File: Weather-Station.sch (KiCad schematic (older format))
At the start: 61 parts

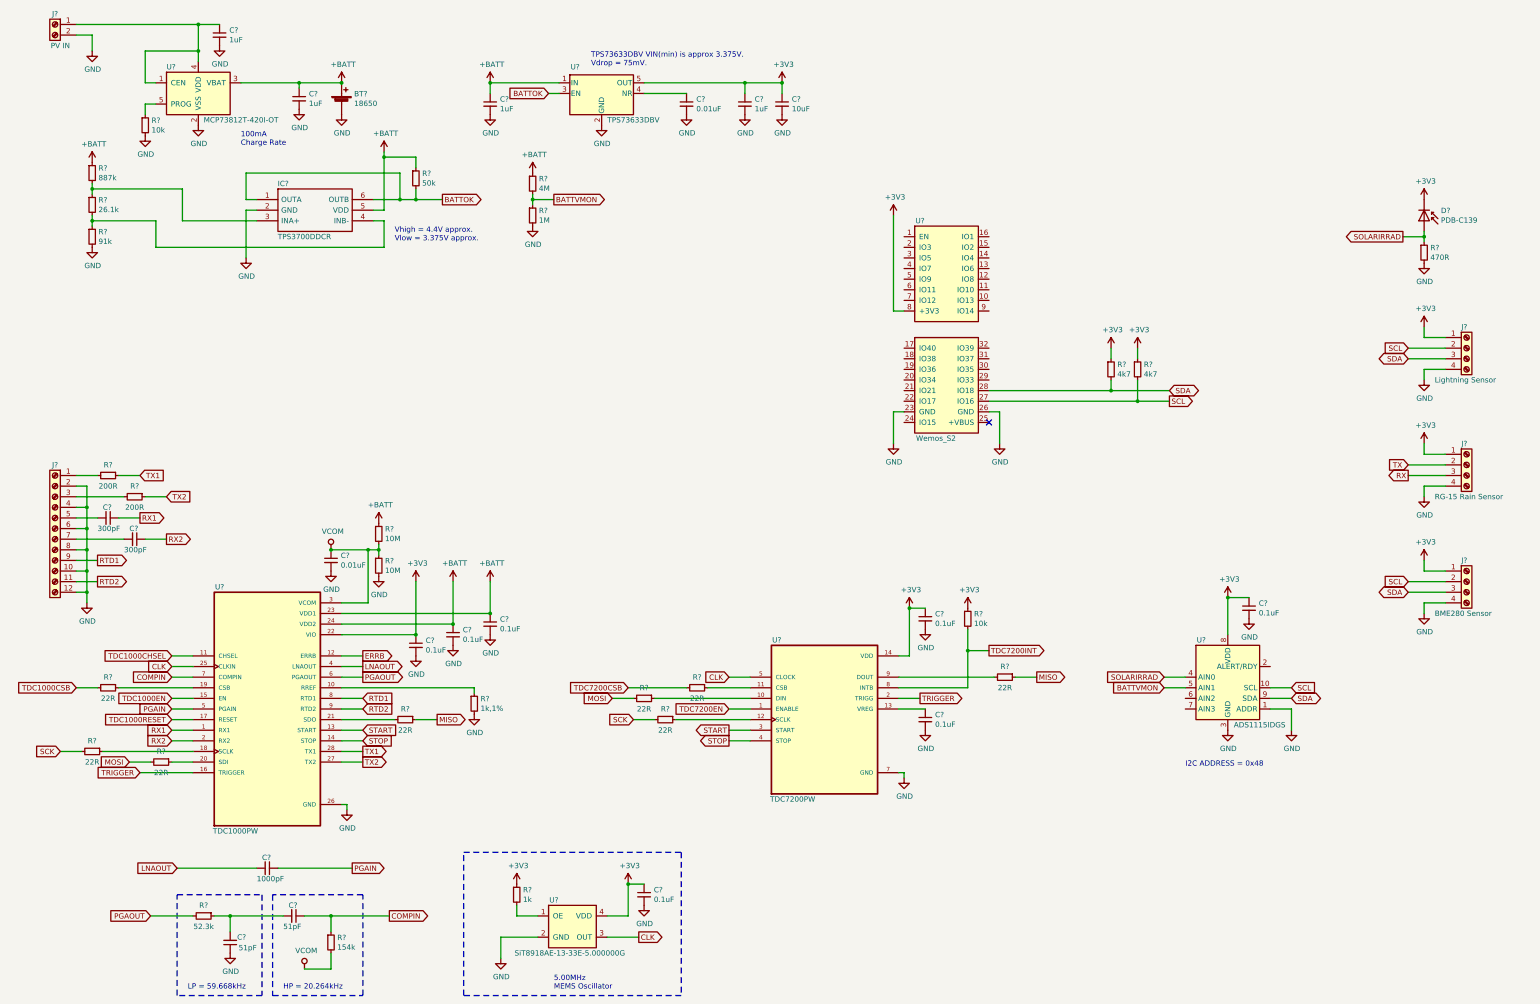
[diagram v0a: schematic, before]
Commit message: Finished schematic
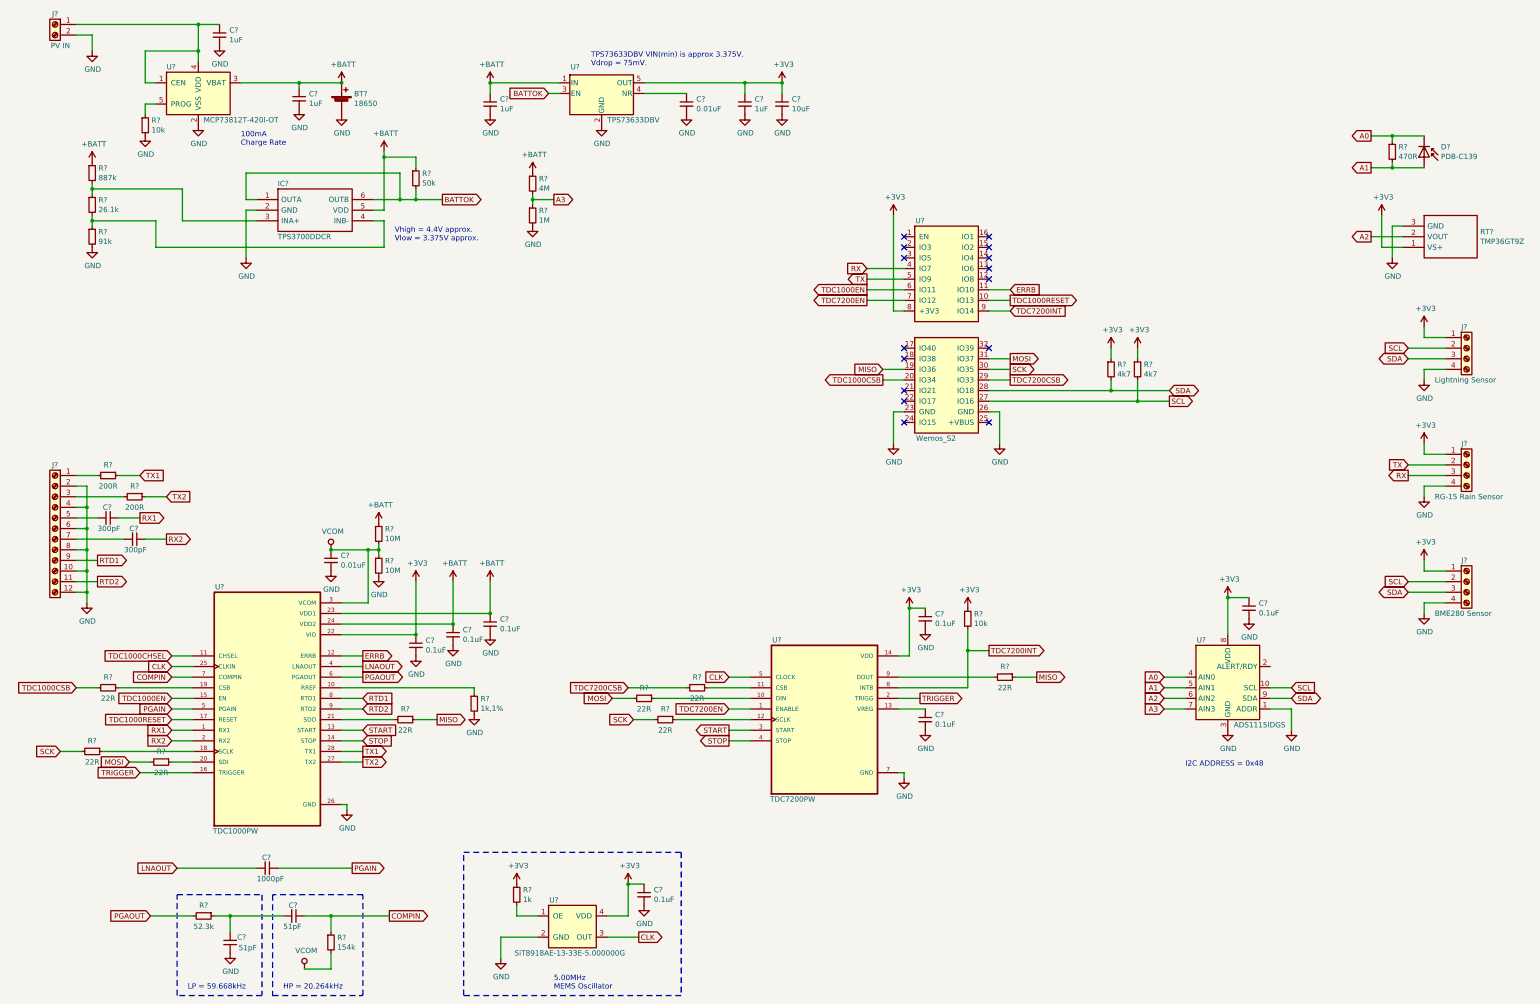
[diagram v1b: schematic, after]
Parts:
- added RT?: TMP36GT9Z, TO-92, symbol TMP36GT9Z:TMP36GT9Z
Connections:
- net +3V3: now also RT?.1 (VS+); no longer D?.1 (K)
- net ERRB: now also U?.11 (IO10)
- net GND: now also RT?.3 (GND); no longer R?.2
- net MISO: now also U?.19 (IO36)
- net MOSI: now also U?.31 (IO37)
- net RX: now also U?.4 (IO7)
- net SCK: now also U?.30 (IO35)
- net TDC1000CSB: now also U?.20 (IO34)
- net TDC1000EN: now also U?.6 (IO11)
- net TDC1000RESET: now also U?.10 (IO13)
- net TDC7200CSB: now also U?.29 (IO33)
- net TDC7200EN: now also U?.7 (IO12)
- net TDC7200INT: now also U?.9 (IO14)
- net TX: now also U?.5 (IO9)
- net A2: now reaches U?.6 (AIN2)
- net A2: now also RT?.2 (VOUT)
- net A3: now reaches U?.7 (AIN3)
- net A3: now also R?.1, R?.2
- removed net BATTVMON: R?.1, R?.2, U?.5 (AIN1)
- net SOLARIRRAD renamed A0
- net A0: now also D?.1 (K); no longer D?.2 (A)
- new net A1: D?.2 (A), R?.2, U?.5 (AIN1)
- no-connect marks 1 -> 15
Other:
- moved on the sheet: D?, R?
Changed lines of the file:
@@
 Text Notes 4500 3350 0    50   ~ 0
 Vhigh = 4.4V approx.\nVlow = 3.375V approx.
-Text GLabel 11750 7550 0    50   Input ~ 0
-BATTVMON
-Text GLabel 6000 2950 2    50   Output ~ 0
-BATTVMON
+Text GLabel 11750 7750 0    50   Input ~ 0
+A3
 $Comp
 L Device:R_Small R?
@@
 L Device:D_Photo D?
 U 1 1 619F7CEC
-P 14200 3150
-F 0 "D?" V 14104 3308 50  0000 L CNN
-F 1 "PDB-C139" V 14195 3308 50  0000 L CNN
-F 2 "" H 14150 3150 50  0001 C CNN
-F 3 "~" H 14150 3150 50  0001 C CNN
-	1    14200 3150
+P 14200 2550
+F 0 "D?" V 14104 2708 50  0000 L CNN
+F 1 "PDB-C139" V 14195 2708 50  0000 L CNN
+F 2 "" H 14150 2550 50  0001 C CNN
+F 3 "~" H 14150 2550 50  0001 C CNN
+	1    14200 2550
 	0    1    1    0
 $EndComp
@@
 L Device:R_Small R?
 U 1 1 619F8699
-P 14200 3450
-F 0 "R?" H 14259 3496 50  0000 L CNN
-F 1 "470R" H 14259 3405 50  0000 L CNN
-F 2 "Resistor_SMD:R_0805_2012Metric" H 14200 3450 50  0001 C CNN
-F 3 "~" H 14200 3450 50  0001 C CNN
-	1    14200 3450
-	1    0    0    -1
-$EndComp
-$Comp
-L power:GND #PWR?
-U 1 1 619F9126
-P 14200 3550
-F 0 "#PWR?" H 14200 3300 50  0001 C CNN
-F 1 "GND" H 14205 3377 50  0000 C CNN
-F 2 "" H 14200 3550 50  0001 C CNN
-F 3 "" H 14200 3550 50  0001 C CNN
-	1    14200 3550
-	1    0    0    -1
-$EndComp
-$Comp
-L power:+3V3 #PWR?
-U 1 1 619F9743
-P 14200 2950
-F 0 "#PWR?" H 14200 2800 50  0001 C CNN
-F 1 "+3V3" H 14215 3123 50  0000 C CNN
-F 2 "" H 14200 2950 50  0001 C CNN
-F 3 "" H 14200 2950 50  0001 C CNN
-	1    14200 2950
-	1    0    0    -1
-$EndComp
-Text GLabel 14000 3300 0    50   Output ~ 0
-SOLARIRRAD
-Wire Wire Line
-	14200 3350 14200 3300
-Wire Wire Line
-	14000 3300 14200 3300
-Connection ~ 14200 3300
-Wire Wire Line
-	14200 3300 14200 3250
+P 13900 2500
+F 0 "R?" H 13959 2546 50  0000 L CNN
+F 1 "470R" H 13959 2455 50  0000 L CNN
+F 2 "Resistor_SMD:R_0805_2012Metric" H 13900 2500 50  0001 C CNN
+F 3 "~" H 13900 2500 50  0001 C CNN
+	1    13900 2500
+	1    0    0    -1
+$EndComp
 $Comp
 L Analog_ADC:ADS1115IDGS U?
@@
 	12350 7050 12350 6700
 Connection ~ 12350 6700
-Text GLabel 11750 7450 0    50   Input ~ 0
-SOLARIRRAD
 Wire Wire Line
 	11750 7450 11950 7450
-Wire Wire Line
-	11750 7550 11950 7550
 Text GLabel 14050 6650 0    50   BiDi ~ 0
 SDA
@@
 Wire Wire Line
 	14200 6750 14200 6850
+Wire Wire Line
+	11750 7750 11950 7750
+Text GLabel 11750 7450 0    50   Input ~ 0
+A0
+Text GLabel 11750 7550 0    50   Input ~ 0
+A1
+Wire Wire Line
+	11950 7550 11750 7550
+Text GLabel 13700 2350 0    50   Output ~ 0
+A0
+Text GLabel 13700 2650 0    50   Output ~ 0
+A1
+Wire Wire Line
+	14200 2650 13900 2650
+Wire Wire Line
+	13900 2650 13900 2600
+Wire Wire Line
+	14200 2350 13900 2350
+Wire Wire Line
+	13900 2350 13900 2400
+Wire Wire Line
+	13700 2350 13900 2350
+Connection ~ 13900 2350
+Wire Wire Line
+	13700 2650 13900 2650
+Connection ~ 13900 2650
+$Comp
+L TMP36GT9Z:TMP36GT9Z RT?
+U 1 1 61B2AD8B
+P 14000 3200
+F 0 "RT?" H 14728 3146 50  0000 L CNN
+F 1 "TMP36GT9Z" H 14728 3055 50  0000 L CNN
+F 2 "TO-92" H 14750 3300 50  0001 L CNN
+F 3 "https://datasheet.datasheetarchive.com/originals/distributors/SFDatasheet-4/sf-00085637.pdf" H 14750 3200 50  0001 L CNN
+F 4 "TMP36GT9Z, Temperature Sensor +/-3C Serial-2 Wire 2.7  5.5 V 3-Pin TO-92" H 14750 3100 50  0001 L CNN "Description"
+F 5 "" H 14750 3000 50  0001 L CNN "Height"
+F 6 "Analog Devices" H 14750 2900 50  0001 L CNN "Manufacturer_Name"
+F 7 "TMP36GT9Z" H 14750 2800 50  0001 L CNN "Manufacturer_Part_Number"
+F 8 "584-TMP36GT9Z" H 14750 2700 50  0001 L CNN "Mouser Part Number"
+F 9 "https://www.mouser.co.uk/ProductDetail/Analog-Devices/TMP36GT9Z?qs=WIvQP4zGanhT97N47MSoHw%3D%3D" H 14750 2600 50  0001 L CNN "Mouser Price/Stock"
+F 10 "TMP36GT9Z" H 14750 2500 50  0001 L CNN "Arrow Part Number"
+F 11 "https://www.arrow.com/en/products/tmp36gt9z/analog-devices?region=nac" H 14750 2400 50  0001 L CNN "Arrow Price/Stock"
+	1    14000 3200
+	1    0    0    -1
+$EndComp
+$Comp
+L power:GND #PWR?
+U 1 1 61B2C44F
+P 13900 3500
+F 0 "#PWR?" H 13900 3250 50  0001 C CNN
+F 1 "GND" H 13905 3327 50  0000 C CNN
+F 2 "" H 13900 3500 50  0001 C CNN
+F 3 "" H 13900 3500 50  0001 C CNN
+	1    13900 3500
+	1    0    0    -1
+$EndComp
+Wire Wire Line
+	13900 3500 13900 3200
+Wire Wire Line
+	13900 3200 14000 3200
+Text GLabel 11750 7650 0    50   Input ~ 0
+A2
+Text GLabel 13700 3300 0    50   Output ~ 0
+A2
+Wire Wire Line
+	13700 3300 14000 3300
+$Comp
+L power:+3V3 #PWR?
+U 1 1 61B45FB8
+P 13800 3100
+F 0 "#PWR?" H 13800 2950 50  0001 C CNN
+F 1 "+3V3" H 13815 3273 50  0000 C CNN
+F 2 "" H 13800 3100 50  0001 C CNN
+F 3 "" H 13800 3100 50  0001 C CNN
+	1    13800 3100
+	1    0    0    -1
+$EndComp
+Wire Wire Line
+	14000 3400 13800 3400
+Wire Wire Line
+	13800 3400 13800 3100
+Wire Wire Line
+	11950 7650 11750 7650
+Text GLabel 6000 2950 2    50   Output ~ 0
+A3
+Wire Wire Line
+	9300 3600 8950 3600
+Wire Wire Line
+	8950 3700 9300 3700
+Text GLabel 8950 3700 0    50   Output ~ 0
+TX
+Text GLabel 8950 3600 0    50   Input ~ 0
+RX
+Text GLabel 9100 4550 0    50   Input ~ 0
+MISO
+Text GLabel 10300 4450 2    50   Output ~ 0
+MOSI
+Text GLabel 10300 4550 2    50   Output ~ 0
+SCK
+Text GLabel 9100 4650 0    50   Output ~ 0
+TDC1000CSB
+Text GLabel 10300 4650 2    50   Output ~ 0
+TDC7200CSB
+Text GLabel 8950 3800 0    50   Output ~ 0
+TDC1000EN
+Text GLabel 8950 3900 0    50   Output ~ 0
+TDC7200EN
+Text GLabel 10300 3900 2    50   Output ~ 0
+TDC1000RESET
+Text GLabel 10300 3800 2    50   Input ~ 0
+ERRB
+Text GLabel 10300 4000 2    50   Input ~ 0
+TDC7200INT
+Wire Wire Line
+	10300 4650 10100 4650
+Wire Wire Line
+	10300 4550 10100 4550
+Wire Wire Line
+	10300 4450 10100 4450
+Wire Wire Line
+	9300 4550 9100 4550
+Wire Wire Line
+	9300 4650 9100 4650
+Wire Wire Line
+	10300 3800 10100 3800
+Wire Wire Line
+	10300 3900 10100 3900
+Wire Wire Line
+	10300 4000 10100 4000
+Wire Wire Line
+	9300 3800 8950 3800
+Wire Wire Line
+	8950 3900 9300 3900
+NoConn ~ 9300 3300
+NoConn ~ 9300 3400
+NoConn ~ 9300 3500
+NoConn ~ 10100 3300
+NoConn ~ 10100 3400
+NoConn ~ 10100 3500
+NoConn ~ 10100 3600
+NoConn ~ 10100 3700
+NoConn ~ 10100 4350
+NoConn ~ 9300 4350
+NoConn ~ 9300 4450
+NoConn ~ 9300 4750
+NoConn ~ 9300 4850
+NoConn ~ 9300 5050
 $EndSCHEMATC
